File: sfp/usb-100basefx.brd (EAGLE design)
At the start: 54 x 29 mm, 52 parts, among them IC1 LD33, IC2 93LC66SN, U1 AX88772BSP, U2 SFP, Y1 25MHz

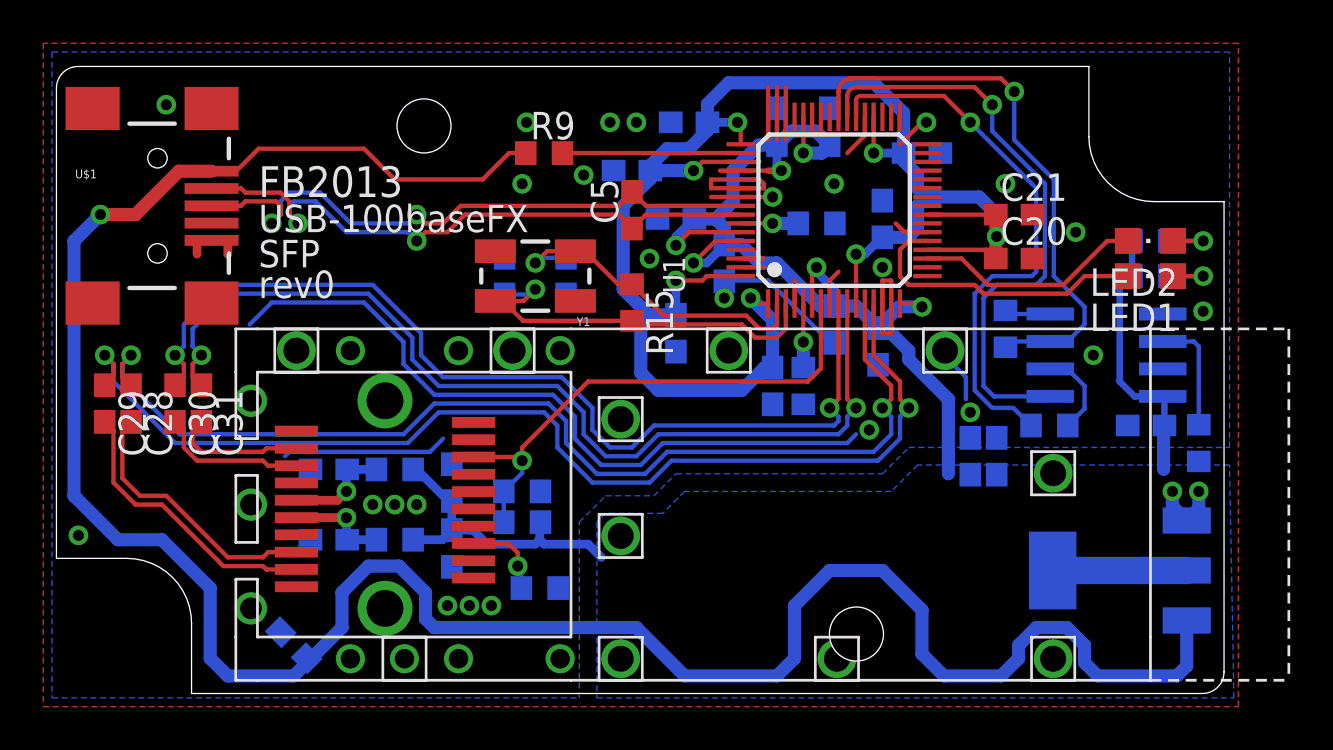
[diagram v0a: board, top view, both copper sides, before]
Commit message: sfp: fixes
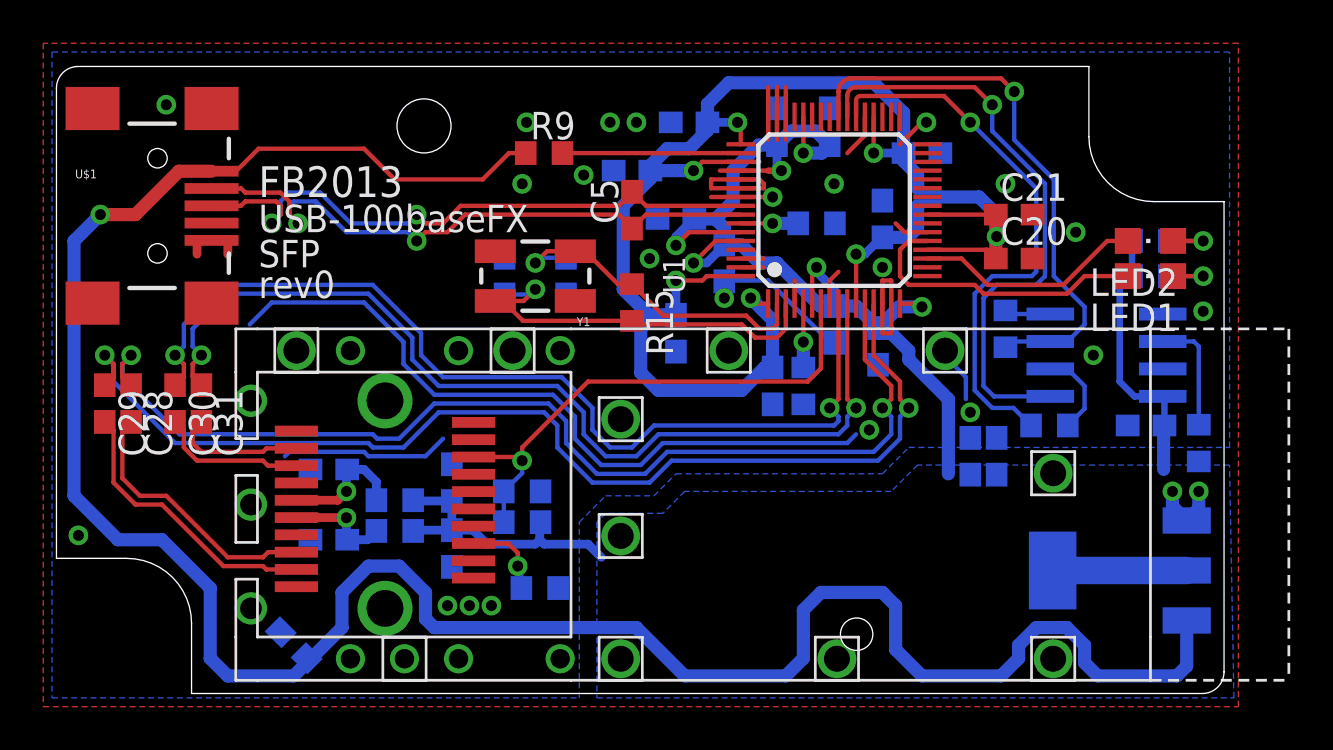
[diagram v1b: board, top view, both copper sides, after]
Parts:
- BOX1: value HAMMOND-BOX-H -> HAMMOND-BOX-H-1H; device hammond:1551H -> hammond:1551H-1HOLE
- moved R1 1.42 mm to (15.6, 8.94)
- moved R3 0.41 mm to (15.6, 7.52)
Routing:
- net VCCR: track 4.86 -> 5.95 mm
- net USB_VIN: track 110.1 -> 109.2 mm
- net VCC: track 84.0 -> 83.2 mm
- net GND: track 86.1 -> 86.2 mm, vias 27 -> 24
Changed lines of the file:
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@@
 <layer number="27" name="tValues" color="7" fill="1" visible="no" active="yes"/>
 <layer number="28" name="bValues" color="7" fill="1" visible="no" active="yes"/>
-<layer number="29" name="tStop" color="7" fill="3" visible="yes" active="yes"/>
+<layer number="29" name="tStop" color="7" fill="3" visible="no" active="yes"/>
 <layer number="30" name="bStop" color="7" fill="6" visible="no" active="yes"/>
 <layer number="31" name="tCream" color="7" fill="4" visible="no" active="yes"/>
@@
 <text x="9.3472" y="19.7104" size="1.27" layer="121">SFP</text>
 <text x="9.3472" y="18.288" size="1.27" layer="121">rev0</text>
+<hole x="37.0078" y="2.7432" drill="1.5"/>
 </plain>
 <attributes>
@@
 <element name="U$1" library="SparkFun-Connectors" package="USB-MINIB" value="USB-MINIB-5PIN" x="4.6736" y="22.5552"/>
 <element name="U1" library="balto" package="LQFP64-0.4MM-SHORTPAD" value="AX88772BSP" x="35.9664" y="22.352"/>
-<element name="BOX1" library="hammond" package="1551H" value="HAMMOND-BOX-H" x="0" y="0" locked="yes"/>
+<element name="BOX1" library="hammond" package="1551H-1HOLE" value="HAMMOND-BOX-H-1H" x="0" y="0" locked="yes"/>
 <element name="C2" library="rcl" package="C0603" value="1u" x="12.5984" y="7.112" rot="MR0"/>
 <element name="C5" library="rcl" package="C0603" value="3p3" x="26.6192" y="22.352" rot="R90"/>
@@
 <element name="C30" library="rcl" package="C0603" value="1u" x="5.4864" y="13.4112" rot="R270"/>
 <element name="C31" library="rcl" package="C0603" value="1u" x="6.7056" y="13.4112" rot="R270"/>
-<element name="R1" library="rcl" package="R0603" value="0" x="15.6464" y="10.3632" rot="MR0"/>
-<element name="R3" library="rcl" package="R0603" value="0" x="15.6464" y="7.112" rot="MR0"/>
+<element name="R1" library="rcl" package="R0603" value="0" x="15.6464" y="8.9408" rot="MR0"/>
+<element name="R3" library="rcl" package="R0603" value="0" x="15.6464" y="7.5184" rot="MR0"/>
 </elements>
 <signals>
@@
 <contactref element="R1" pad="1"/>
 <contactref element="C12" pad="1"/>
-<wire x1="16.4964" y1="10.3632" x2="16.6624" y2="10.3632" width="0.4064" layer="16"/>
-<wire x1="16.6624" y1="10.3632" x2="18.122" y2="8.9036" width="0.4064" layer="16"/>
-<wire x1="18.288" y1="8.9036" x2="18.122" y2="8.9036" width="0.4064" layer="16"/>
-<wire x1="16.4964" y1="7.112" x2="17.8444" y2="7.112" width="0.4064" layer="16"/>
-<wire x1="17.8444" y1="7.112" x2="18.288" y2="7.5556" width="0.4064" layer="16"/>
 <wire x1="18.288" y1="8.9036" x2="18.288" y2="7.5556" width="0.4064" layer="16"/>
 <wire x1="18.288" y1="7.5556" x2="19.2668" y2="7.5556" width="0.4064" layer="16"/>
@@
 <wire x1="41.2496" y1="13.6144" x2="41.2496" y2="10.16" width="0.6096" layer="16"/>
 <wire x1="49.7468" y1="20.9296" x2="49.7468" y2="19.304" width="0.3048" layer="16"/>
+<wire x1="18.288" y1="7.5556" x2="16.5336" y2="7.5556" width="0.4064" layer="16"/>
+<wire x1="16.5336" y1="7.5556" x2="16.4964" y2="7.5184" width="0.4064" layer="16"/>
+<wire x1="18.288" y1="8.9036" x2="16.5336" y2="8.9036" width="0.4064" layer="16"/>
+<wire x1="16.5336" y1="8.9036" x2="16.4964" y2="8.9408" width="0.4064" layer="16"/>
 </signal>
 <signal name="GND">
@@
 <wire x1="28.0416" y1="11.5824" x2="36.576" y2="11.5824" width="0.2032" layer="16"/>
 <wire x1="36.576" y1="11.5824" x2="36.9824" y2="11.9888" width="0.2032" layer="16"/>
-<via x="14.6304" y="8.7376" extent="1-16" drill="0.508"/>
-<via x="16.6624" y="8.7376" extent="1-16" drill="0.508"/>
-<via x="15.6464" y="8.7376" extent="1-16" drill="0.508"/>
 <wire x1="14.224" y1="18.0848" x2="16.0528" y2="16.256" width="0.2032" layer="16"/>
-<wire x1="10.7696" y1="11.176" x2="17.272" y2="11.176" width="0.2032" layer="16"/>
+<wire x1="10.7696" y1="11.176" x2="14.224" y2="11.176" width="0.2032" layer="16"/>
+<wire x1="14.224" y1="11.176" x2="14.4272" y2="10.9728" width="0.2032" layer="16"/>
+<wire x1="14.4272" y1="10.9728" x2="17.0688" y2="10.9728" width="0.2032" layer="16"/>
 <wire x1="10.7696" y1="11.176" x2="10.5664" y2="10.9728" width="0.2032" layer="16"/>
-<wire x1="17.272" y1="11.176" x2="17.8816" y2="11.7856" width="0.2032" layer="16"/>
+<wire x1="17.0688" y1="10.9728" x2="17.8816" y2="11.7856" width="0.2032" layer="16"/>
 <via x="18.0848" y="4.064" extent="1-16" drill="0.508"/>
 <via x="19.1008" y="4.064" extent="1-16" drill="0.508"/>
@@
 <wire x1="42.0624" y1="13.6144" x2="42.0624" y2="14.6304" width="0.2032" layer="16"/>
 <wire x1="42.0624" y1="14.6304" x2="41.2496" y2="15.4432" width="0.2032" layer="16"/>
-<wire x1="36.576" y1="11.5824" x2="36.0968" y2="1.6076" width="0" layer="19" extent="16-16"/>
 </signal>
 <signal name="TD_DP">
@@
 <wire x1="3.048" y1="15.24" x2="3.4544" y2="15.6464" width="0.2032" layer="16"/>
 <wire x1="22.7584" y1="13.4112" x2="17.4752" y2="13.4112" width="0.2032" layer="16"/>
-<wire x1="17.4752" y1="13.4112" x2="16.0528" y2="11.9888" width="0.2032" layer="16"/>
-<wire x1="16.0528" y1="11.9888" x2="5.6896" y2="11.9888" width="0.2032" layer="16"/>
+<wire x1="17.4752" y1="13.4112" x2="15.8496" y2="11.7856" width="0.2032" layer="16"/>
+<wire x1="15.8496" y1="11.7856" x2="14.8336" y2="11.7856" width="0.2032" layer="16"/>
+<wire x1="14.8336" y1="11.7856" x2="14.6304" y2="11.9888" width="0.2032" layer="16"/>
+<wire x1="14.6304" y1="11.9888" x2="5.6896" y2="11.9888" width="0.2032" layer="16"/>
 <wire x1="5.6896" y1="11.9888" x2="3.048" y2="14.6304" width="0.2032" layer="16"/>
 </signal>
@@
 <wire x1="2.6416" y1="15.24" x2="2.2352" y2="15.6464" width="0.2032" layer="16"/>
 <wire x1="22.5552" y1="13.0048" x2="17.6784" y2="13.0048" width="0.2032" layer="16"/>
-<wire x1="17.6784" y1="13.0048" x2="16.256" y2="11.5824" width="0.2032" layer="16"/>
-<wire x1="16.256" y1="11.5824" x2="5.4864" y2="11.5824" width="0.2032" layer="16"/>
+<wire x1="17.6784" y1="13.0048" x2="16.0528" y2="11.3792" width="0.2032" layer="16"/>
+<wire x1="16.0528" y1="11.3792" x2="14.6304" y2="11.3792" width="0.2032" layer="16"/>
+<wire x1="14.6304" y1="11.3792" x2="14.4272" y2="11.5824" width="0.2032" layer="16"/>
+<wire x1="14.4272" y1="11.5824" x2="5.4864" y2="11.5824" width="0.2032" layer="16"/>
 <wire x1="5.4864" y1="11.5824" x2="2.6416" y2="14.4272" width="0.2032" layer="16"/>
 </signal>
@@
 <wire x1="17.4752" y1="3.048" x2="26.8224" y2="3.048" width="0.6096" layer="16"/>
 <wire x1="26.8224" y1="3.048" x2="29.0576" y2="0.8128" width="0.6096" layer="16"/>
-<wire x1="29.0576" y1="0.8128" x2="33.3248" y2="0.8128" width="0.6096" layer="16"/>
-<wire x1="33.3248" y1="0.8128" x2="34.1376" y2="1.6256" width="0.6096" layer="16"/>
-<wire x1="34.1376" y1="1.6256" x2="34.1376" y2="4.064" width="0.6096" layer="16"/>
-<wire x1="34.1376" y1="4.064" x2="35.7632" y2="5.6896" width="0.6096" layer="16"/>
-<wire x1="35.7632" y1="5.6896" x2="38.2016" y2="5.6896" width="0.6096" layer="16"/>
-<wire x1="38.2016" y1="5.6896" x2="40.0304" y2="3.8608" width="0.6096" layer="16"/>
-<wire x1="40.0304" y1="3.8608" x2="40.0304" y2="1.8288" width="0.6096" layer="16"/>
-<wire x1="40.0304" y1="1.8288" x2="41.0464" y2="0.8128" width="0.6096" layer="16"/>
-<wire x1="41.0464" y1="0.8128" x2="43.688" y2="0.8128" width="0.6096" layer="16"/>
+<wire x1="29.0576" y1="0.8128" x2="33.7312" y2="0.8128" width="0.6096" layer="16"/>
+<wire x1="33.7312" y1="0.8128" x2="34.544" y2="1.6256" width="0.6096" layer="16"/>
+<wire x1="34.544" y1="1.6256" x2="34.544" y2="3.8608" width="0.6096" layer="16"/>
+<wire x1="34.544" y1="3.8608" x2="35.3568" y2="4.6736" width="0.6096" layer="16"/>
+<wire x1="35.3568" y1="4.6736" x2="38.2016" y2="4.6736" width="0.6096" layer="16"/>
+<wire x1="38.2016" y1="4.6736" x2="38.8112" y2="4.064" width="0.6096" layer="16"/>
+<wire x1="38.8112" y1="4.064" x2="38.8112" y2="2.032" width="0.6096" layer="16"/>
+<wire x1="38.8112" y1="2.032" x2="40.0304" y2="0.8128" width="0.6096" layer="16"/>
+<wire x1="40.0304" y1="0.8128" x2="43.688" y2="0.8128" width="0.6096" layer="16"/>
 <wire x1="43.688" y1="0.8128" x2="44.5008" y2="1.6256" width="0.6096" layer="16"/>
 <wire x1="44.5008" y1="1.6256" x2="44.5008" y2="2.2352" width="0.6096" layer="16"/>
@@
 <wire x1="13.4112" y1="9.3472" x2="13.4112" y2="10.326" width="0.4064" layer="16"/>
 <wire x1="13.4112" y1="10.326" x2="13.4484" y2="10.3632" width="0.4064" layer="16"/>
-<wire x1="13.4484" y1="10.3632" x2="14.7964" y2="10.3632" width="0.4064" layer="16"/>
+<wire x1="13.4484" y1="10.3632" x2="14.224" y2="10.3632" width="0.4064" layer="16"/>
+<wire x1="14.224" y1="10.3632" x2="14.7964" y2="9.7908" width="0.4064" layer="16"/>
+<wire x1="14.7964" y1="8.9408" x2="14.7964" y2="9.7908" width="0.4064" layer="16"/>
 </signal>
 <signal name="VCCT">
@@
 <wire x1="13.4112" y1="8.128" x2="13.4112" y2="7.1492" width="0.4064" layer="16"/>
 <wire x1="13.4112" y1="7.1492" x2="13.4484" y2="7.112" width="0.4064" layer="16"/>
-<wire x1="13.4484" y1="7.112" x2="14.7964" y2="7.112" width="0.4064" layer="16"/>
+<wire x1="13.4484" y1="7.112" x2="14.39" y2="7.112" width="0.4064" layer="16"/>
+<wire x1="14.39" y1="7.112" x2="14.7964" y2="7.5184" width="0.4064" layer="16"/>
 </signal>
 </signals>
